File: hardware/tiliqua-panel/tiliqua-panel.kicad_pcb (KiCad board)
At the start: 2 copper layers, 30 x 128.5 mm, 17 parts

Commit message: * apf.audio + nlnet on panel
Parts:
- added G***: LOGO, LOGO, F.Cu at (19.0, 121.2)
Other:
- board text added: "[apf.audio]"
- board text removed: "[apfelaudio]"

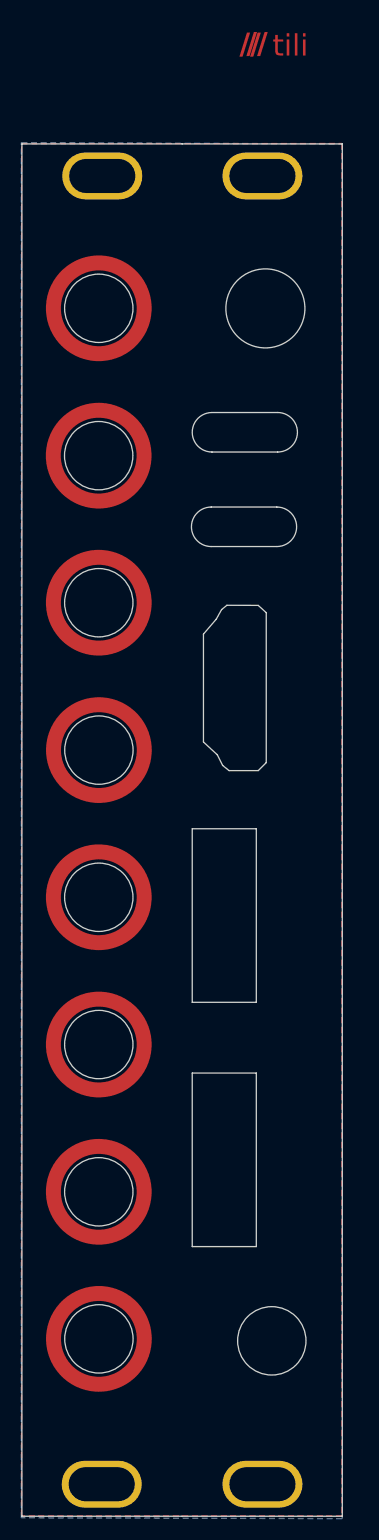
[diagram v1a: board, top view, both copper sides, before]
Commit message: * fab 05.01.24
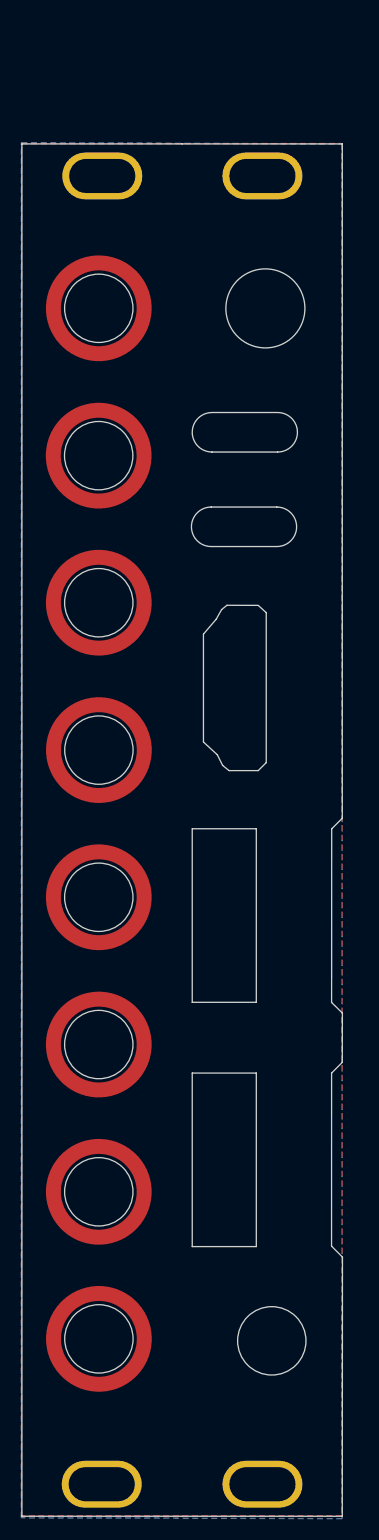
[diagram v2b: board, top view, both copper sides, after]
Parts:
- moved G*** 14.6 mm to (25.8, 58.5)
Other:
- outline, holes or cut-outs redrawn
- board text added: "gpdi"
- board text removed: "//"
- board text removed: "dvi"
- board text removed: "qua"
- board text removed: "tili"
